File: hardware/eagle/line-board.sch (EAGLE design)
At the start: 34 parts

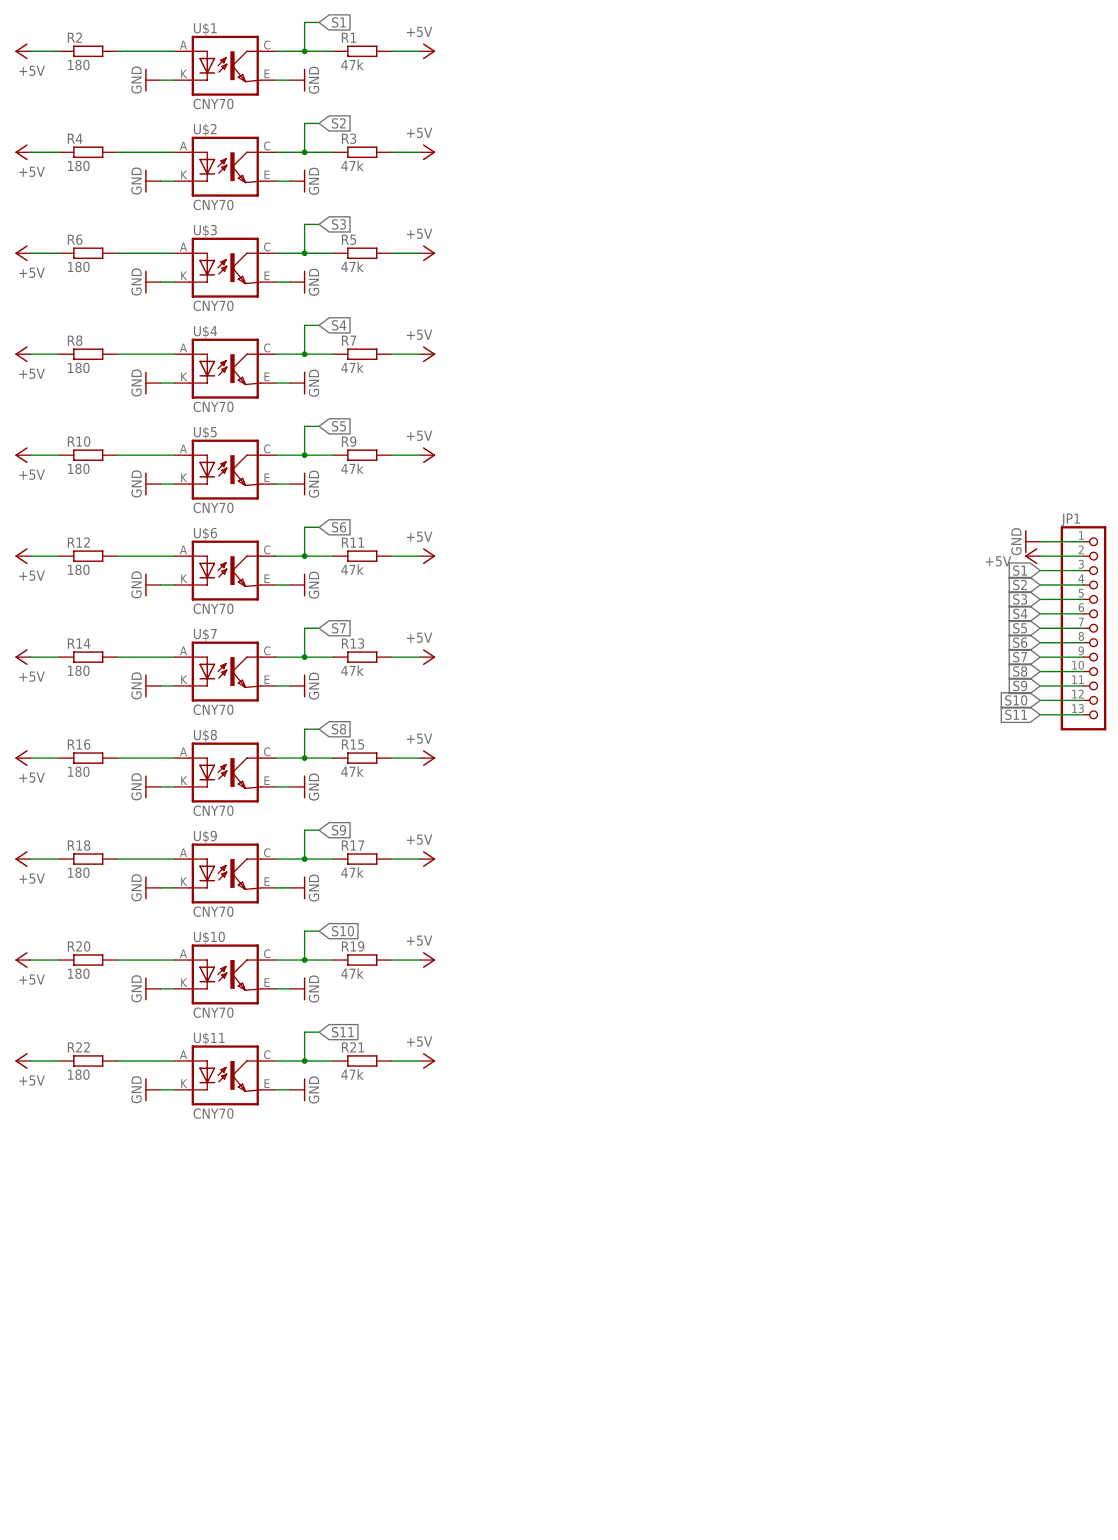
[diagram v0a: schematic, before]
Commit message: layout
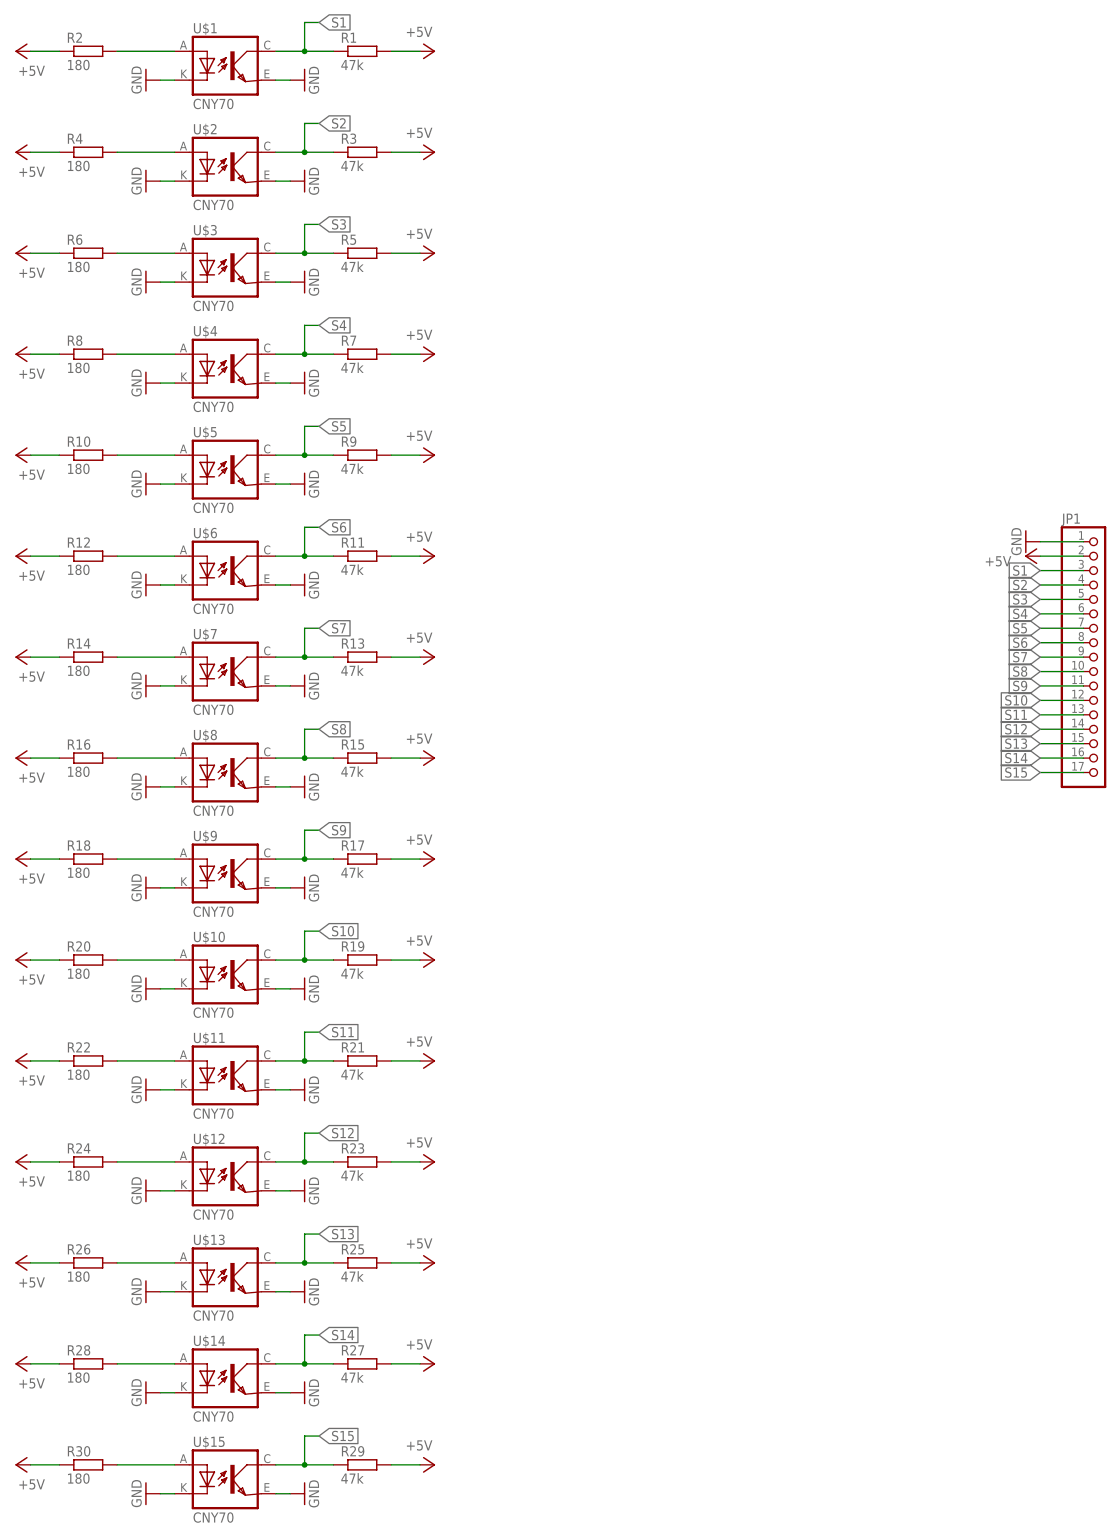
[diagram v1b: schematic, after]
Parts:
- added R23, R25, R27, R29: 47k, rcl:R-EU_R1206
- added R24, R26, R28, R30: 180, rcl:R-EU_R1206
- added U$12, U$13, U$14, U$15: CNY70, cny70:CNY70
- JP1: device pinhead:PINHD-1X13 -> pinhead:PINHD-1X17
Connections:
- new net N$1: R24.2, U$12.A
- new net N$4: R26.2, U$13.A
- new net N$6: R28.2, U$14.A
- new net N$8: R30.2, U$15.A
- new net S12: JP1.14, R23.1, U$12.COL
- new net S13: JP1.15, R25.1, U$13.COL
- new net S14: JP1.16, R27.1, U$14.COL
- new net S15: JP1.17, R29.1, U$15.COL
- net +5V: now also R23.2, R24.1, R25.2, R26.1, R27.2, R28.1, R29.2, R30.1
- net GND: now also U$12.C, U$12.EMI, U$13.C, U$13.EMI, U$14.C, U$14.EMI, U$15.C, U$15.EMI

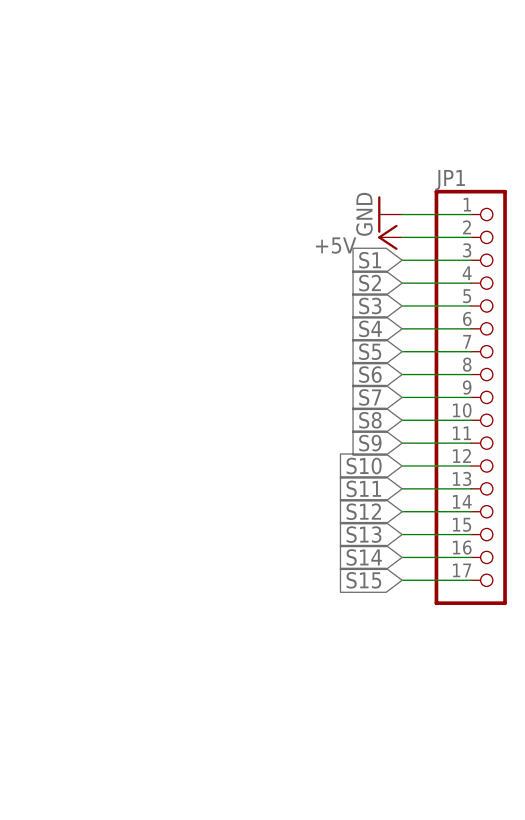
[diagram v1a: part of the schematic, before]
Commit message: hw version 1.0.0
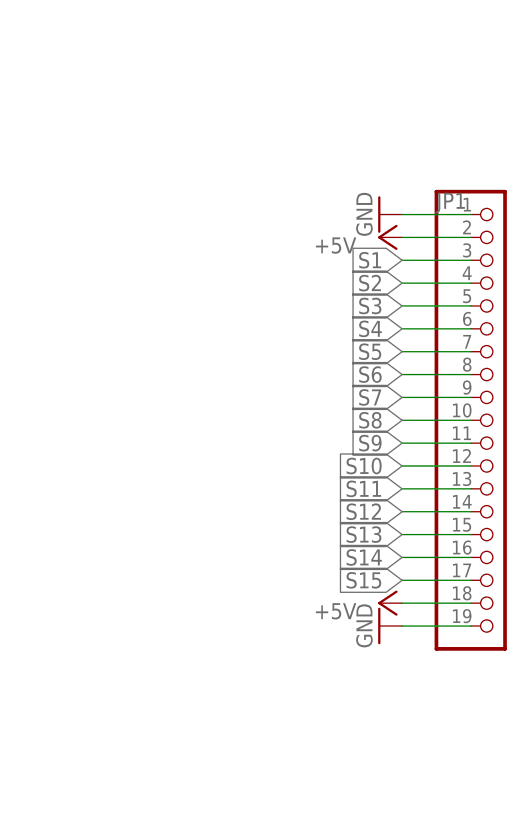
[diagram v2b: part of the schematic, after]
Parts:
- JP1: device pinhead:PINHD-1X17 -> pinhead:PINHD-1X19
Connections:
- net +5V: now also JP1.18
- net GND: now also JP1.19
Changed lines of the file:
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@@
 <part name="P+30" library="supply1" library_urn="urn:adsk.eagle:library:371" deviceset="+5V" device=""/>
 <part name="P+31" library="supply1" library_urn="urn:adsk.eagle:library:371" deviceset="+5V" device=""/>
-<part name="JP1" library="pinhead" library_urn="urn:adsk.eagle:library:325" deviceset="PINHD-1X17" device="" package3d_urn="urn:adsk.eagle:package:22490/2"/>
+<part name="JP1" library="pinhead" library_urn="urn:adsk.eagle:library:325" deviceset="PINHD-1X19" device="" package3d_urn="urn:adsk.eagle:package:22492/2"/>
+<part name="GND32" library="supply1" library_urn="urn:adsk.eagle:library:371" deviceset="GND" device=""/>
+<part name="P+32" library="supply1" library_urn="urn:adsk.eagle:library:371" deviceset="+5V" device=""/>
 </parts>
 <sheets>
@@
 <attribute name="VALUE" x="7.62" y="-121.92" size="1.778" layer="96" rot="R180"/>
 </instance>
-<instance part="JP1" gate="G$1" x="193.04" y="-27.94" smashed="yes">
-<attribute name="NAME" x="186.69" y="-6.985" size="1.778" layer="95"/>
-<attribute name="VALUE" x="186.69" y="-55.88" size="1.778" layer="96"/>
+<instance part="JP1" gate="G$1" x="193.04" y="-30.48" smashed="yes">
+<attribute name="NAME" x="186.69" y="-9.525" size="1.778" layer="95"/>
+<attribute name="VALUE" x="186.69" y="-58.42" size="1.778" layer="96"/>
+</instance>
+<instance part="GND32" gate="1" x="180.34" y="-55.88" smashed="yes" rot="R270">
+<attribute name="VALUE" x="177.8" y="-53.34" size="1.778" layer="96" rot="R270"/>
+</instance>
+<instance part="P+32" gate="1" x="180.34" y="-53.34" smashed="yes" rot="R90">
+<attribute name="VALUE" x="177.8" y="-53.34" size="1.778" layer="96" rot="R180"/>
 </instance>
 </instances>
@@
 <wire x1="182.88" y1="-10.16" x2="190.5" y2="-10.16" width="0.1524" layer="91"/>
 </segment>
+<segment>
+<pinref part="GND32" gate="1" pin="GND"/>
+<pinref part="JP1" gate="G$1" pin="19"/>
+<wire x1="182.88" y1="-55.88" x2="190.5" y2="-55.88" width="0.1524" layer="91"/>
+</segment>
 </net>
 <net name="N$2" class="0">
@@
 <wire x1="182.88" y1="-12.7" x2="190.5" y2="-12.7" width="0.1524" layer="91"/>
 </segment>
-</net>
+<segment>
+<pinref part="P+32" gate="1" pin="+5V"/>
+<pinref part="JP1" gate="G$1" pin="18"/>
+<wire x1="182.88" y1="-53.34" x2="190.5" y2="-53.34" width="0.1524" layer="91"/>
+</segment>
+</net>
